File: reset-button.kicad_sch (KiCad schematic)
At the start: 3 parts, among them SW1 KMR2

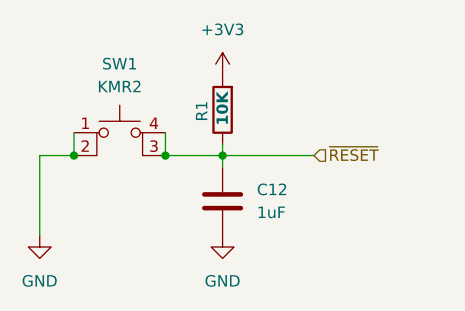
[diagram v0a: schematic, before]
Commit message: Starting layout
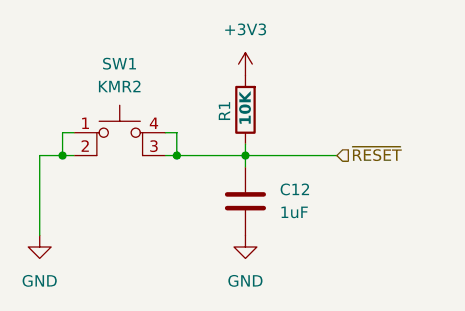
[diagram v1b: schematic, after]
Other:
- moved on the sheet: C12, R1
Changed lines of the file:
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@@
 	)
 	(junction
-		(at 153.67 97.79)
+		(at 156.21 97.79)
 		(diameter 0)
 		(color 0 0 0 0)
 	)
 	(junction
-		(at 137.16 97.79)
+		(at 135.89 97.79)
 		(diameter 0)
 		(color 0 0 0 0)
 	)
 	(junction
-		(at 147.32 97.79)
+		(at 148.59 97.79)
 		(diameter 0)
 		(color 0 0 0 0)
@@
 	(wire
 		(pts
-			(xy 153.67 97.79) (xy 153.67 99.06)
-		)
-		(stroke
-			(width 0)
-			(type default)
-		)
-	)
-	(wire
-		(pts
-			(xy 137.16 95.25) (xy 137.16 97.79)
+			(xy 156.21 97.79) (xy 156.21 99.06)
+		)
+		(stroke
+			(width 0)
+			(type default)
+		)
+	)
+	(wire
+		(pts
+			(xy 135.89 97.79) (xy 137.16 97.79)
+		)
+		(stroke
+			(width 0)
+			(type default)
+		)
+	)
+	(wire
+		(pts
+			(xy 133.35 97.79) (xy 135.89 97.79)
 		)
 		(stroke
@@
 	(wire
 		(pts
-			(xy 147.32 95.25) (xy 147.32 97.79)
-		)
-		(stroke
-			(width 0)
-			(type default)
-		)
-	)
-	(wire
-		(pts
-			(xy 147.32 97.79) (xy 153.67 97.79)
-		)
-		(stroke
-			(width 0)
-			(type default)
-		)
-	)
-	(wire
-		(pts
-			(xy 153.67 97.79) (xy 163.83 97.79)
-		)
-		(stroke
-			(width 0)
-			(type default)
-		)
-	)
-	(wire
-		(pts
-			(xy 133.35 97.79) (xy 137.16 97.79)
-		)
-		(stroke
-			(width 0)
-			(type default)
-		)
-	)
-	(wire
-		(pts
-			(xy 153.67 97.79) (xy 153.67 96.52)
+			(xy 148.59 95.25) (xy 148.59 97.79)
+		)
+		(stroke
+			(width 0)
+			(type default)
+		)
+	)
+	(wire
+		(pts
+			(xy 135.89 95.25) (xy 135.89 97.79)
+		)
+		(stroke
+			(width 0)
+			(type default)
+		)
+	)
+	(wire
+		(pts
+			(xy 156.21 97.79) (xy 166.37 97.79)
+		)
+		(stroke
+			(width 0)
+			(type default)
+		)
+	)
+	(wire
+		(pts
+			(xy 147.32 97.79) (xy 148.59 97.79)
+		)
+		(stroke
+			(width 0)
+			(type default)
+		)
+	)
+	(wire
+		(pts
+			(xy 148.59 95.25) (xy 147.32 95.25)
+		)
+		(stroke
+			(width 0)
+			(type default)
+		)
+	)
+	(wire
+		(pts
+			(xy 156.21 97.79) (xy 156.21 96.52)
+		)
+		(stroke
+			(width 0)
+			(type default)
+		)
+	)
+	(wire
+		(pts
+			(xy 148.59 97.79) (xy 156.21 97.79)
+		)
+		(stroke
+			(width 0)
+			(type default)
+		)
+	)
+	(wire
+		(pts
+			(xy 137.16 95.25) (xy 135.89 95.25)
 		)
 		(stroke
@@
 	(hierarchical_label "~{RESET}"
 		(shape input)
-		(at 163.83 97.79 0)
+		(at 166.37 97.79 0)
 		(fields_autoplaced yes)
 		(effects
@@
 	(symbol
 		(lib_id "Device:C")
-		(at 153.67 102.87 0)
+		(at 156.21 102.87 0)
 		(unit 1)
 		(exclude_from_sim no)
@@
 		(fields_autoplaced yes)
 		(property "Reference" "C12"
-			(at 157.48 101.5999 0)
+			(at 160.02 101.5999 0)
 			(effects
 				(font
@@
 		)
 		(property "Value" "1uF"
-			(at 157.48 104.1399 0)
+			(at 160.02 104.1399 0)
 			(effects
 				(font
@@
 		)
 		(property "Footprint" "Capacitor_SMD:C_0603_1608Metric"
-			(at 154.6352 106.68 0)
+			(at 157.1752 106.68 0)
 			(effects
 				(font
@@
 		)
 		(property "Datasheet" "https://www.yageo.com/upload/media/product/productsearch/datasheet/mlcc/UPY-GPHC_X7R_6"
-			(at 153.67 102.87 0)
+			(at 156.21 102.87 0)
 			(effects
 				(font
@@
 		)
 		(property "Description" "1 uF 10% 16V Ceramic Capacitor X7R 0603 (1608 Metric)"
-			(at 153.67 102.87 0)
+			(at 156.21 102.87 0)
 			(effects
 				(font
@@
 		)
 		(property "Mfr" "YAGEO"
-			(at 153.67 102.87 0)
+			(at 156.21 102.87 0)
 			(effects
 				(font
@@
 		)
 		(property "Mfr P/N" "CC0603KRX7R7BB105"
-			(at 153.67 102.87 0)
+			(at 156.21 102.87 0)
 			(effects
 				(font
@@
 		)
 		(property "Supplier_1" "Digikey"
-			(at 153.67 102.87 0)
+			(at 156.21 102.87 0)
 			(effects
 				(font
@@
 		)
 		(property "Supplier_1 P/N" "0.10"
-			(at 153.67 102.87 0)
+			(at 156.21 102.87 0)
 			(effects
 				(font
@@
 		)
 		(property "Supplier_1 Unit Price" "0.03080"
-			(at 153.67 102.87 0)
+			(at 156.21 102.87 0)
 			(effects
 				(font
@@
 		)
 		(property "Supplier_1 Price @ Qty" ""
-			(at 153.67 102.87 0)
+			(at 156.21 102.87 0)
 			(effects
 				(font
@@
 		)
 		(property "Supplier_2" ""
-			(at 153.67 102.87 0)
+			(at 156.21 102.87 0)
 			(effects
 				(font
@@
 		)
 		(property "Supplier_2 P/N" ""
-			(at 153.67 102.87 0)
+			(at 156.21 102.87 0)
 			(effects
 				(font
@@
 		)
 		(property "Supplier_2 Unit Price" ""
-			(at 153.67 102.87 0)
+			(at 156.21 102.87 0)
 			(effects
 				(font
@@
 		)
 		(property "Supplier_2 Price @ Qty" ""
-			(at 153.67 102.87 0)
+			(at 156.21 102.87 0)
 			(effects
 				(font
@@
 	(symbol
 		(lib_id "Device:R")
-		(at 153.67 92.71 180)
+		(at 156.21 92.71 180)
 		(unit 1)
 		(exclude_from_sim no)
@@
 		(dnp no)
 		(property "Reference" "R1"
-			(at 151.384 91.694 90)
+			(at 153.924 91.694 90)
 			(effects
 				(font
@@
 		)
 		(property "Value" "10K"
-			(at 153.67 90.678 90)
+			(at 156.21 90.678 90)
 			(effects
 				(font
@@
 		)
 		(property "Footprint" "Resistor_SMD:R_0603_1608Metric"
-			(at 155.448 92.71 90)
+			(at 157.988 92.71 90)
 			(effects
 				(font
@@
 		)
 		(property "Datasheet" "https://www.seielect.com/catalog/sei-rncp.pdf"
-			(at 153.67 92.71 0)
+			(at 156.21 92.71 0)
 			(effects
 				(font
@@
 		)
 		(property "Description" "10 kOhms 1% 0.125W, 1/8W Chip Resistor 0603 (1608 Metric) Anti-Sulfur Thin Film"
-			(at 153.67 92.71 0)
+			(at 156.21 92.71 0)
 			(effects
 				(font
@@
 		)
 		(property "Mfr" "Stackpole Electronics Inc"
-			(at 153.67 92.71 0)
+			(at 156.21 92.71 0)
 			(effects
 				(font
@@
 		)
 		(property "Mfr P/N" "RNCP0603FTD10K0"
-			(at 153.67 92.71 0)
+			(at 156.21 92.71 0)
 			(effects
 				(font
@@
 		)
 		(property "Supplier_1" "Digikey"
-			(at 153.67 92.71 0)
+			(at 156.21 92.71 0)
 			(effects
 				(font
@@
 		)
 		(property "Supplier_1 P/N" "RNCP0603FTD10K0CT-ND"
-			(at 153.67 92.71 0)
+			(at 156.21 92.71 0)
 			(effects
 				(font
@@
 		)
 		(property "Supplier_1 Unit Price" "0.10"
-			(at 153.67 92.71 0)
+			(at 156.21 92.71 0)
 			(effects
 				(font
@@
 		)
 		(property "Supplier_1 Price @ Qty" "0.0170"
-			(at 153.67 92.71 0)
+			(at 156.21 92.71 0)
 			(effects
 				(font
@@
 		)
 		(property "Supplier_2" ""
-			(at 153.67 92.71 0)
+			(at 156.21 92.71 0)
 			(effects
 				(font
@@
 		)
 		(property "Supplier_2 P/N" ""
-			(at 153.67 92.71 0)
+			(at 156.21 92.71 0)
 			(effects
 				(font
@@
 		)
 		(property "Supplier_2 Unit Price" ""
-			(at 153.67 92.71 0)
+			(at 156.21 92.71 0)
 			(effects
 				(font
@@
 		)
 		(property "Supplier_2 Price @ Qty" ""
-			(at 153.67 92.71 0)
+			(at 156.21 92.71 0)
 			(effects
 				(font
@@
 	(symbol
 		(lib_id "power:+3V3")
-		(at 153.67 88.9 0)
+		(at 156.21 88.9 0)
 		(unit 1)
 		(exclude_from_sim no)
@@
 		(fields_autoplaced yes)
 		(property "Reference" "#PWR03"
-			(at 153.67 92.71 0)
+			(at 156.21 92.71 0)
 			(effects
 				(font
@@
 		)
 		(property "Value" "+3V3"
-			(at 153.67 83.82 0)
+			(at 156.21 83.82 0)
 			(effects
 				(font
@@
 		)
 		(property "Footprint" ""
-			(at 153.67 88.9 0)
+			(at 156.21 88.9 0)
 			(effects
 				(font
@@
 		)
 		(property "Datasheet" ""
-			(at 153.67 88.9 0)
+			(at 156.21 88.9 0)
 			(effects
 				(font
@@
 		)
 		(property "Description" "Power symbol creates a global label with name \"+3V3\""
-			(at 153.67 88.9 0)
+			(at 156.21 88.9 0)
 			(effects
 				(font
@@
 	(symbol
 		(lib_id "power:GND")
-		(at 153.67 106.68 0)
+		(at 156.21 106.68 0)
 		(unit 1)
 		(exclude_from_sim no)
@@
 		(fields_autoplaced yes)
 		(property "Reference" "#PWR02"
-			(at 153.67 113.03 0)
+			(at 156.21 113.03 0)
 			(effects
 				(font
@@
 		)
 		(property "Value" "GND"
-			(at 153.67 111.76 0)
+			(at 156.21 111.76 0)
 			(effects
 				(font
@@
 		)
 		(property "Footprint" ""
-			(at 153.67 106.68 0)
+			(at 156.21 106.68 0)
 			(effects
 				(font
@@
 		)
 		(property "Datasheet" ""
-			(at 153.67 106.68 0)
+			(at 156.21 106.68 0)
 			(effects
 				(font
@@
 		)
 		(property "Description" "Power symbol creates a global label with name \"GND\" , ground"
-			(at 153.67 106.68 0)
-			(effects
-				(font
+			(at 156.21 106.68 0)
+			(effects
+				(font
